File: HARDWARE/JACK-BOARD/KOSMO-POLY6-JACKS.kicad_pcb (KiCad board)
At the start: 2 copper layers, 70 x 175 mm, 30 parts, among them J1 RAMP_OUT0, J10 RAMP_OUT3, J11 PULSE_OUT3, J12 GATE_OUT3, J13 RAMP_OUT4, J14 PULSE_OUT4, J15 GATE_OUT4, J16 RAMP_OUT5, J17 PULSE_OUT5, J18 GATE_OUT5, J2 PULSE_OUT0, J3 GATE_OUT0, J4 RAMP_OUT1, J5 PULSE_OUT1, J6 GATE_OUT1, J7 RAMP_OUT2, J8 PULSE_OUT2, J9 GATE_OUT2

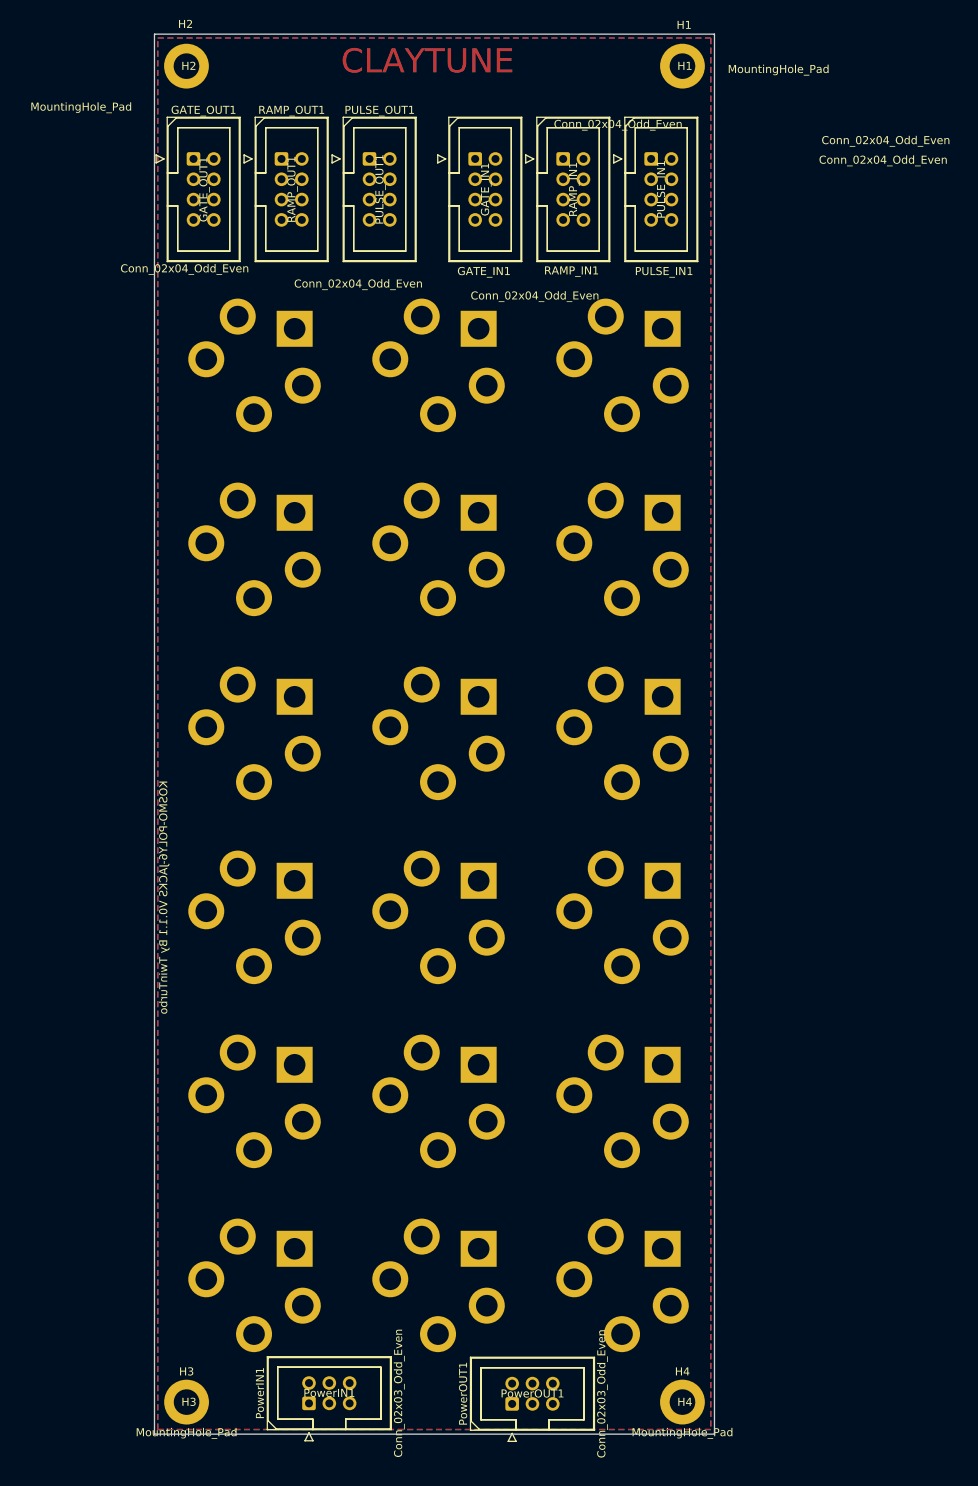
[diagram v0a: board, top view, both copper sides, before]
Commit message: sync
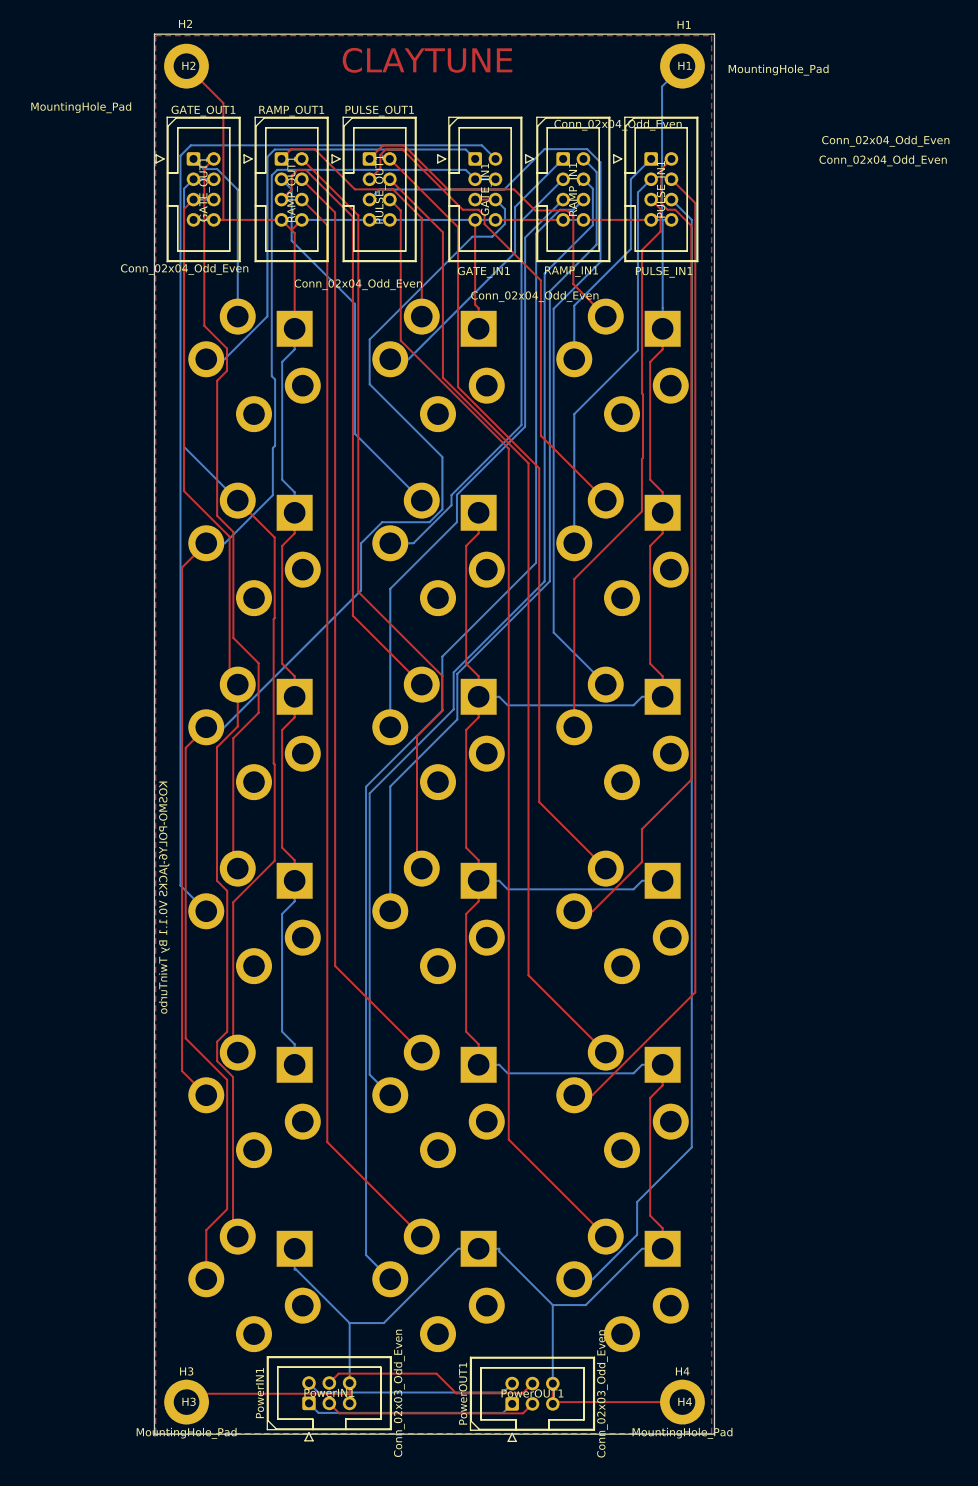
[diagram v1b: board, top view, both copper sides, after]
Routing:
- net GND-S: track 0.00 -> 577.3 mm
- net GATE_OUT2-S: track 0.00 -> 171.5 mm
- net GATE_OUT1-S: track 0.00 -> 151.3 mm
- net RAMP_OUT5-S: track 0.00 -> 148.4 mm
- net PULSE_OUT5-S: track 0.00 -> 143.4 mm
- net PULSE_OUT5-N: track 0.00 -> 140.8 mm
- net GATE_OUT2-N: track 0.00 -> 138.6 mm
- net GATE_OUT3-S: track 0.00 -> 136.4 mm
- net RAMP_OUT5-N: track 0.00 -> 135.8 mm
- net RAMP_OUT4-S: track 0.00 -> 127.6 mm
- net PULSE_OUT4-S: track 0.00 -> 123.3 mm
- net PULSE_OUT4-N: track 0.00 -> 120.3 mm
- net GATE_OUT1-N: track 0.00 -> 119.4 mm
- net RAMP_OUT4-N: track 0.00 -> 115.4 mm
- net RAMP_OUT3-S: track 0.00 -> 105.4 mm
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- removed copper zone on B.Cu, net GND-S

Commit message: Kicad7 and Fixlayered
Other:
- net class Default removed
